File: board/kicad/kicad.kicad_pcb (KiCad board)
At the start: 2 copper layers, 220.5 x 102.5 mm, 24 parts

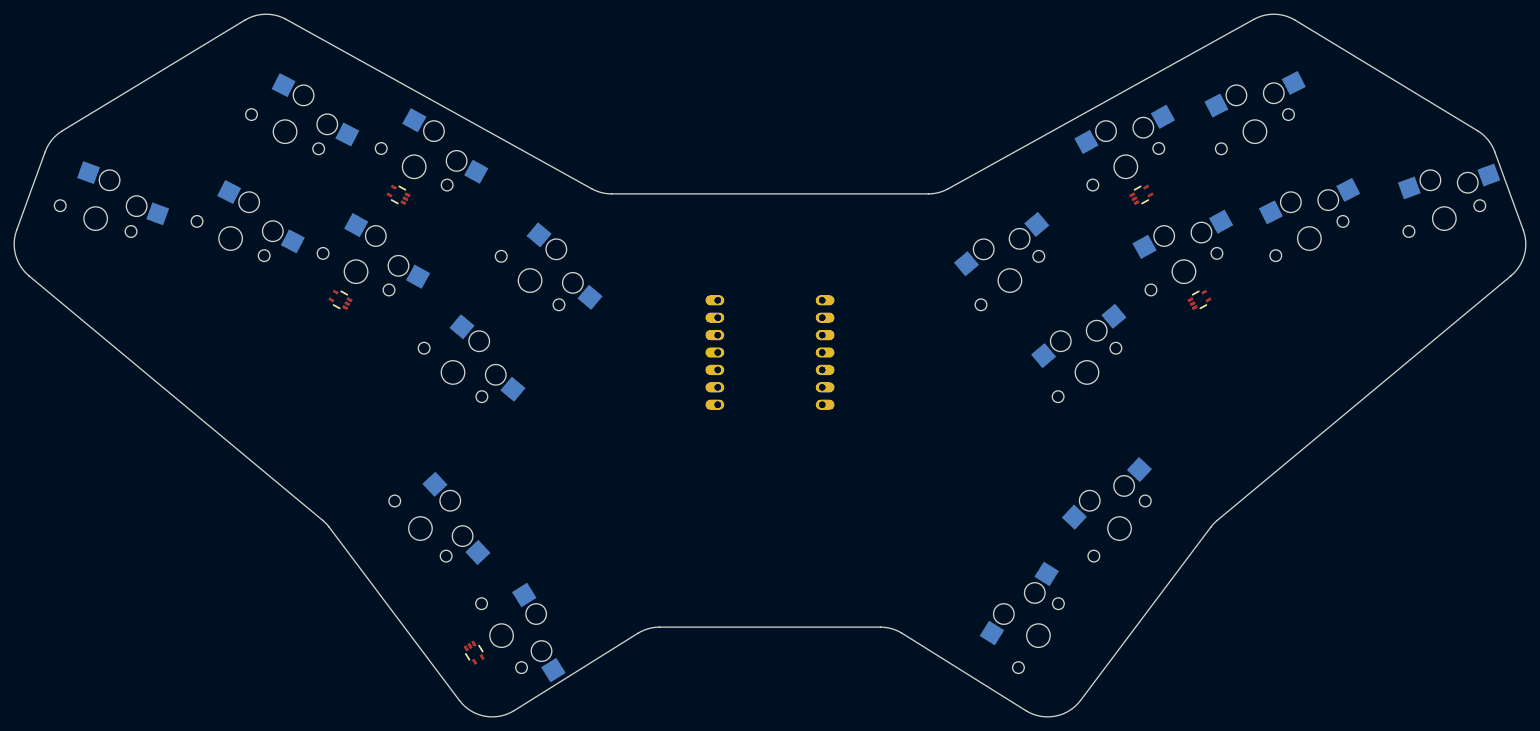
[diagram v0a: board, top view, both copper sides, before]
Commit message: feat: 20 keys
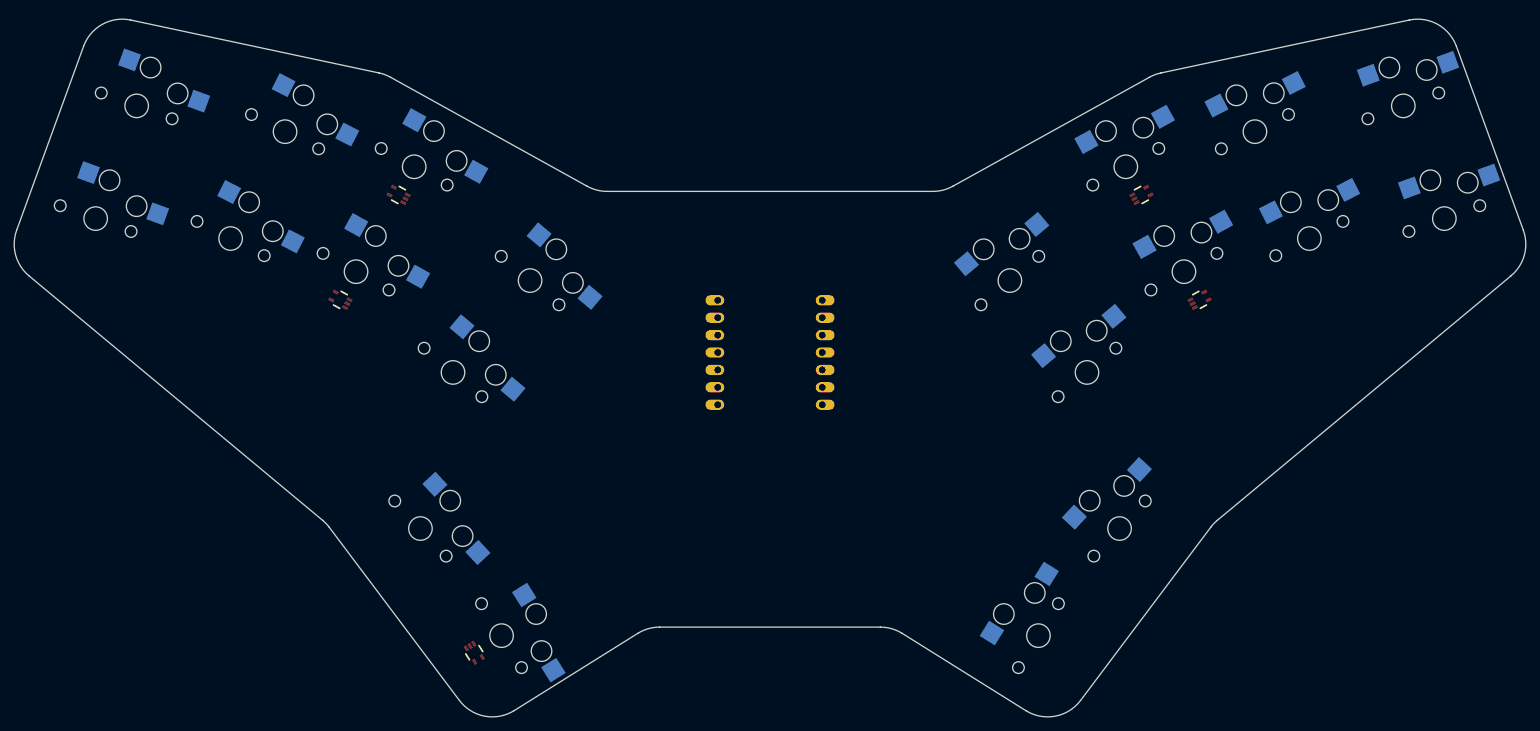
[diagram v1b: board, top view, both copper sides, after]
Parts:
- added S19: , PG1350, F.Cu at (270.5, 212.1)
- added S20: , PG1350, F.Cu at (258.6, 227.7)
- moved S8 133.7 mm to (184.5, 175.9), turned to -40 degrees
- moved S17 102.0 mm to (168.5, 212.1), turned to -47 degrees
- moved S15 99.9 mm to (265.7, 189.3), turned to 40 degrees
- moved S16 90.5 mm to (254.5, 175.9), turned to 40 degrees
- moved S18 78.3 mm to (180.3, 227.7), turned to -58 degrees
- moved S6 30.5 mm to (167.5, 159.3), turned to -29 degrees
- moved S2 23.7 mm to (127.1, 150.4), turned to -20 degrees
- moved S14 23.7 mm to (271.4, 159.3), turned to 29 degrees
- moved S4 22.9 mm to (148.7, 154.2), turned to -27 degrees
- moved S10 22.0 mm to (311.9, 150.4), turned to 20 degrees
- moved S13 20.4 mm to (279.9, 174.6), turned to 29 degrees
- moved S9 19.9 mm to (317.8, 166.9), turned to 20 degrees
- moved S12 19.5 mm to (290.2, 154.2), turned to 27 degrees
- moved S11 18.9 mm to (298.2, 169.8), turned to 27 degrees
- moved S3 17.5 mm to (140.8, 169.8)
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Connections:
- S10 pad 1: mirror_ring_top -> mirror_pinky_top
- S10 pad 2: P2 -> P1
- S11 pad 1: mirror_middle_home -> mirror_ring_home
- S11 pad 2: P7 -> P2
- S12 pad 1: mirror_middle_top -> mirror_ring_top
- S12 pad 2: P7 -> P2
- S13 pad 1: mirror_index_home -> mirror_middle_home
- S13 pad 2: P0 -> P7
- S14 pad 1: mirror_index_top -> mirror_middle_top
- S14 pad 2: P0 -> P7
- S15 pad 1: home_default -> mirror_index_home
- S16 pad 1: outer_default -> mirror_index_top
- S16 pad 2: P7 -> P0
- S17 pad 1: mirror_home_default -> home_default
- S17 pad 2: P1 -> P0
- S18 pad 1: mirror_outer_default -> outer_default
- S18 pad 2: P2 -> P7
- S2 pad 1: ring_home -> pinky_top
- S2 pad 2: P7 -> P0
- S3 pad 1: ring_top -> ring_home
- S4 pad 1: middle_home -> ring_top
- S4 pad 2: P2 -> P7
- S5 pad 1: middle_top -> middle_home
- S6 pad 1: index_home -> middle_top
- S6 pad 2: P1 -> P2
- S7 pad 1: index_top -> index_home
- S8 pad 1: mirror_pinky_home -> index_top
- S9 pad 1: mirror_ring_home -> mirror_pinky_home
- S9 pad 2: P2 -> P1
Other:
- board size 220.5 x 102.5 mm -> 220.5 x 101.8 mm
- net class Default added: clearance 0.2, trace_width 0.25, via_dia 0.8, via_drill 0.4

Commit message: chore: upgrade kicad file version
This is the result of opening the file generated by Ergogen in the
latest kicad version.
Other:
- net class Default removed
